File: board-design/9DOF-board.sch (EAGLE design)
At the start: 13 parts

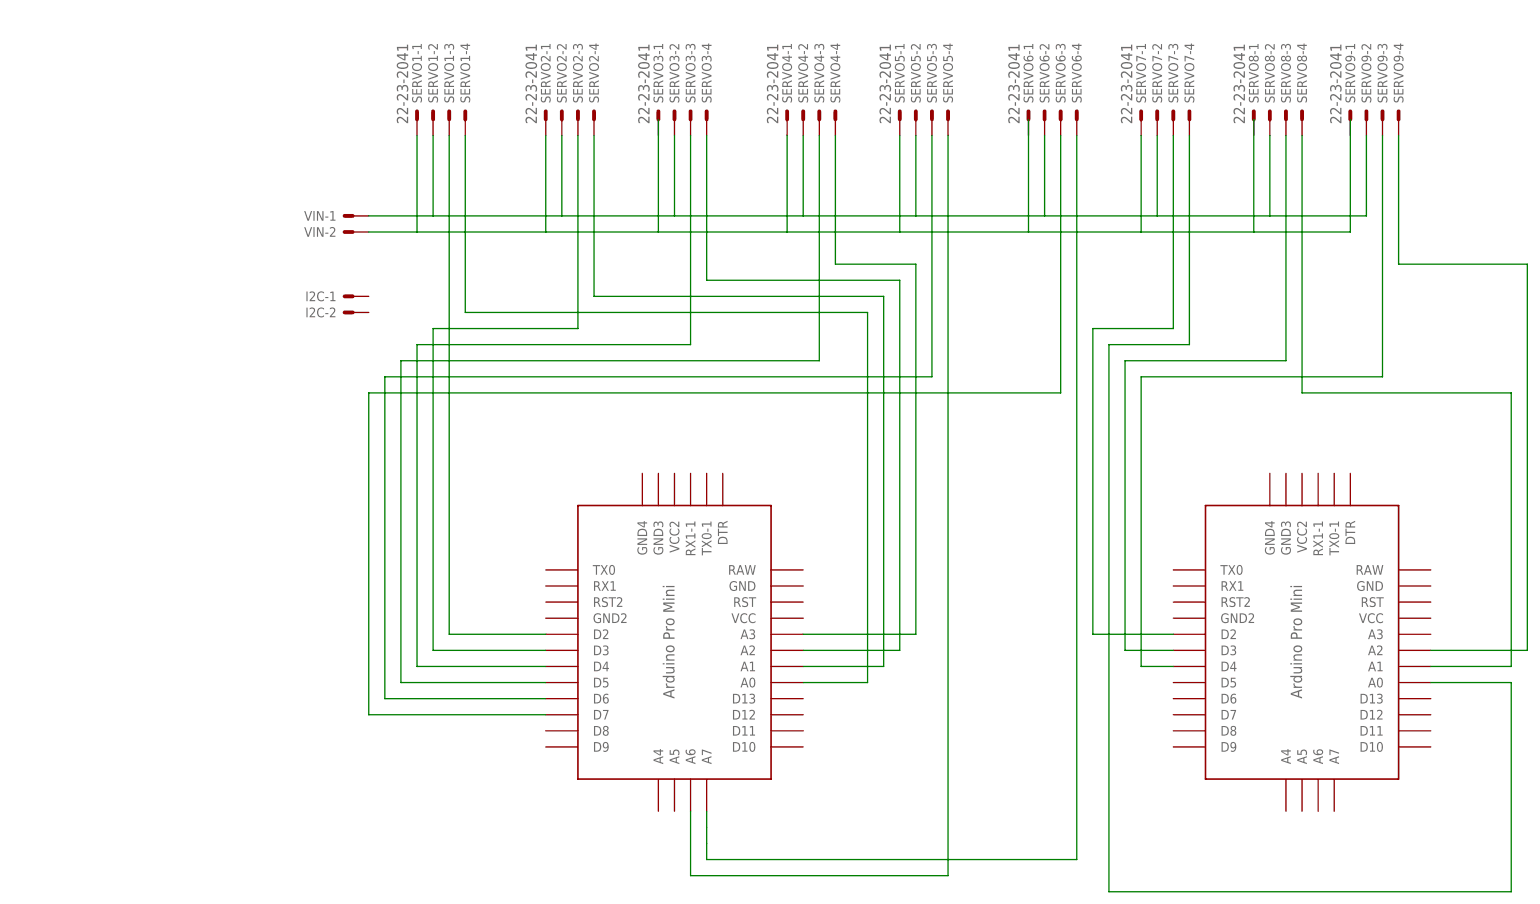
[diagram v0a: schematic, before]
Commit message: Add files via upload
PCB Layout v0.1
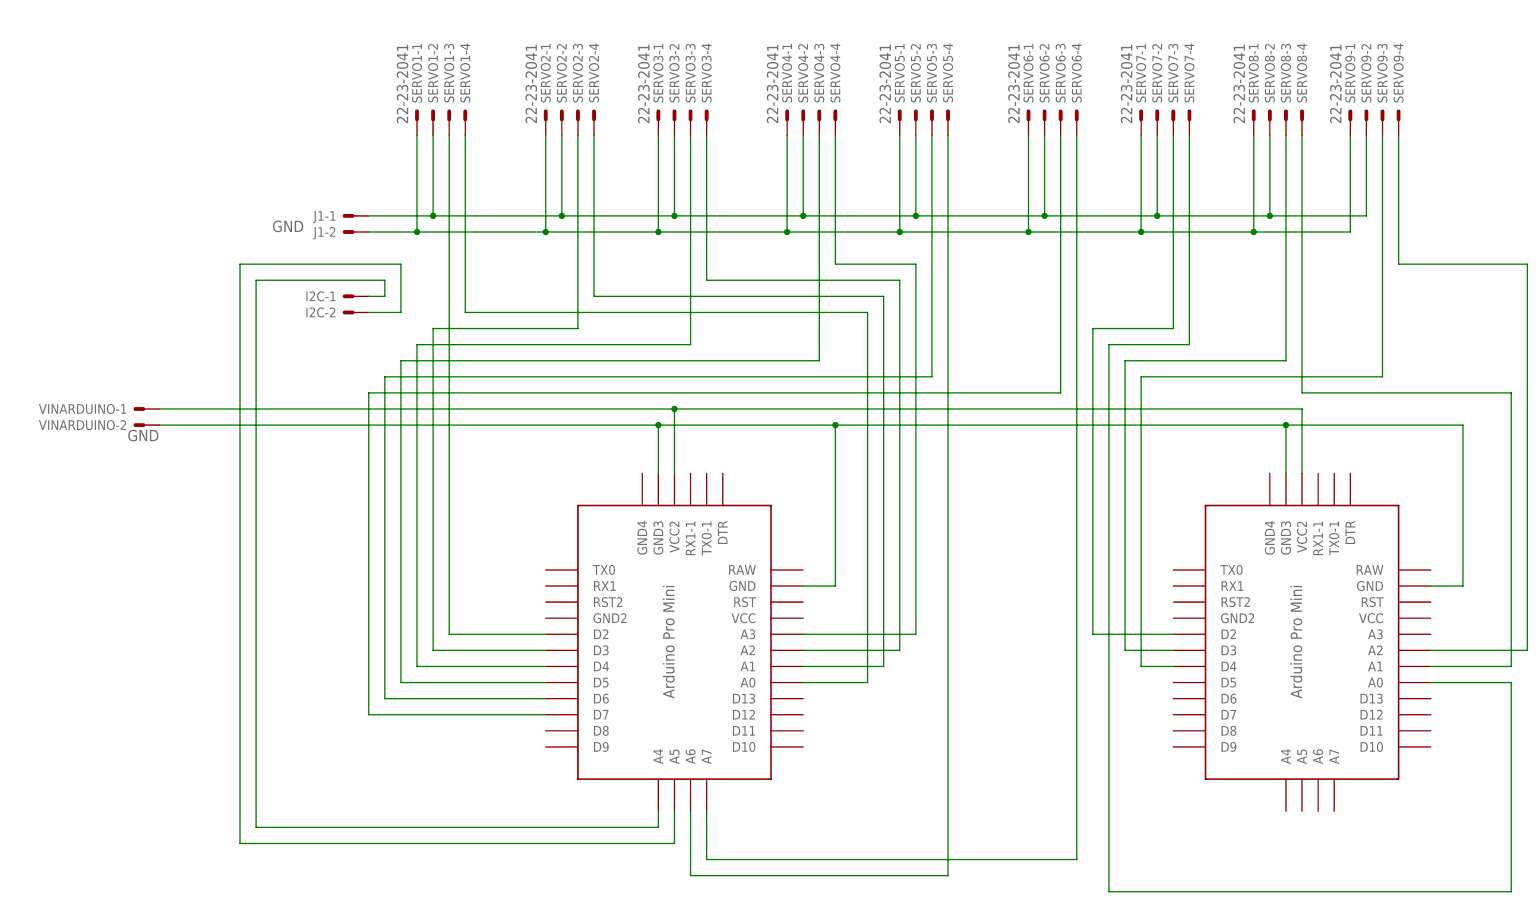
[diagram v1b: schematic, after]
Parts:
- added VINARDUINO: 22-23-2021, con-molex:22-23-2021
- renumbered VIN to J1
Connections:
- net N$1 renamed SERVO1_POT
- net N$10 renamed SERVO9_POT
- net N$11 renamed SERVO6_POT
- net N$12 renamed SERVO2_SIG
- net N$13 renamed SERVO7_POT
- net N$14 renamed SERVO3_SIG
- net N$15 renamed SERVO4_SIG
- net N$16 renamed SERVO5_SIG
- net N$17 renamed SERVO6_SIG
- net N$18 renamed SERVO8_POT
- net N$19 renamed SERVO9_SIG
- net N$2 renamed SERVO2_POT
- net N$20 renamed SERVO7_SIG
- net N$3 renamed SERVO3_POT
- net N$4 renamed SERVO4_POT
- net N$5 renamed SERVO1_SIG
- net N$7 renamed SERVO8_SIG
- net N$8 renamed SERVO5_POT
- net N$9 renamed VCC_SERVO
- removed net N$6: J1-2.S, SERVO1-1.S, SERVO2-1.S, SERVO4-1.S, SERVO5-1.S, SERVO7-1.S
- new net GND: J1-2.S, SERVO1-1.S, SERVO2-1.S, SERVO3-1.S, SERVO4-1.S, SERVO5-1.S, SERVO6-1.S, SERVO7-1.S, SERVO8-1.S, SERVO9-1.S, U$1.GND, U$1.GND3, U$2.GND, U$2.GND3, VINARDUINO-2.S
- new net I2C_SCA: I2C-1.S, U$1.A4
- new net I2C_SCL: I2C-2.S, U$1.A5
- new net VCC_ARDUINO: U$1.VCC2, U$2.VCC2, VINARDUINO-1.S
